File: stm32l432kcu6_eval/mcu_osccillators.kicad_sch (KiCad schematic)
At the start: 8 parts, among them U1 STM32L432KCUx, Y1 ASFL1-40.000MHZ-EC-T, Y2 FC-135_32.7680KA-A3

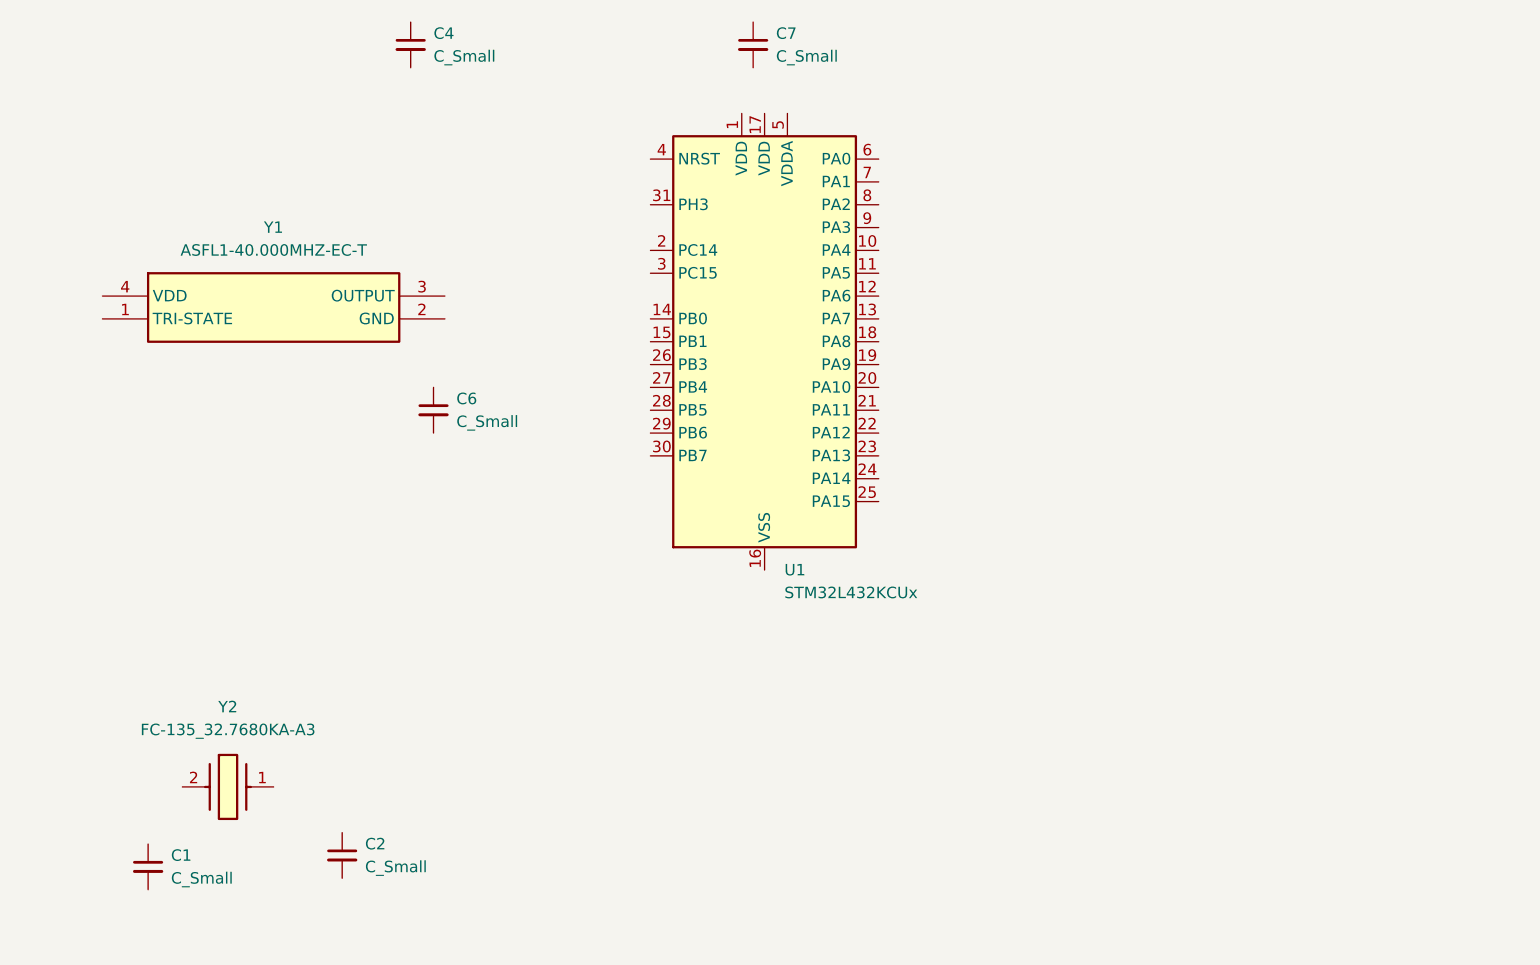
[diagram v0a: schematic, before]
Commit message: board save 1
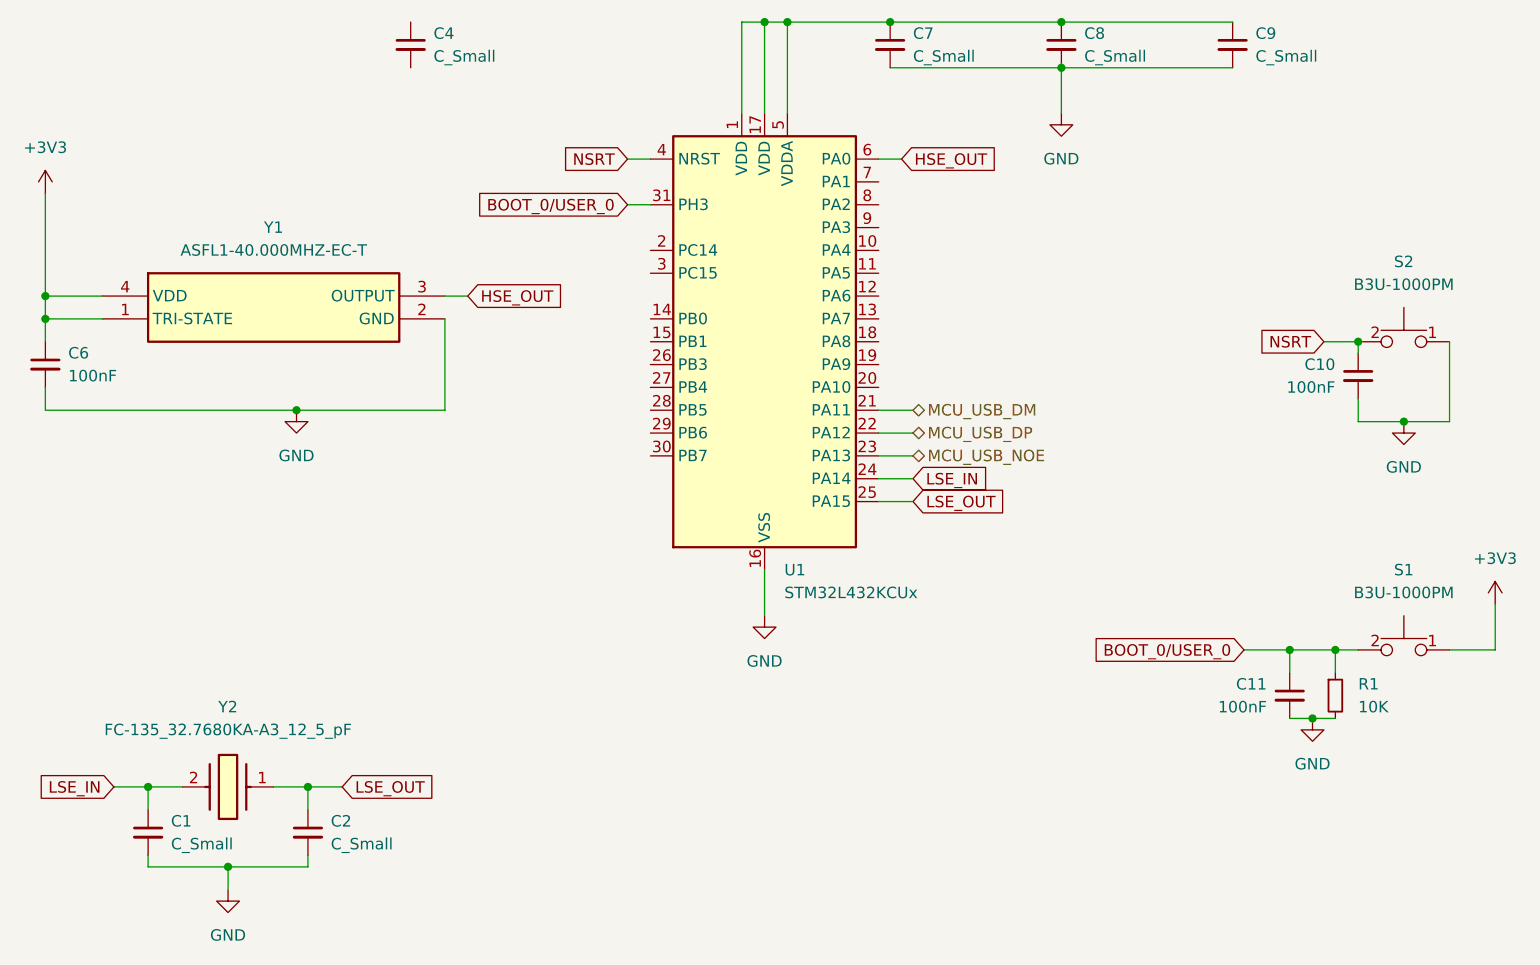
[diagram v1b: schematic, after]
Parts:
- added C10, C11: 100nF, Capacitor_SMD:C_0603_1608Metric, symbol Device:C_Small
- added C8, C9: C_Small, Capacitor_SMD:C_0603_1608Metric, symbol Device:C_Small
- added R1: 10K, Resistor_SMD:R_0603_1608Metric, symbol Device:R_Small
- added S1, S2: B3U-1000PM, custom_part_library_1:B3U1000PM_3D_MODEL, symbol B3U-1000PM_OMRON:B3U-1000PM
- C6: value C_Small -> 100nF
- Y2: value FC-135_32.7680KA-A3 -> FC-135_32.7680KA-A3_12_5_pF
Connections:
- net at U1.1 (VDD): now also C7.1, U1.17 (VDD), U1.5 (VDDA), C8.1, C9.1
- net GND: now reaches U1.16 (VSS), U1.32 (VSS), U1.33 (VSS)
- net GND: now also C1.2, C2.2, C6.2, C7.2, Y1.2 (GND), C10.2, C11.2, C8.2, C9.2, R1.2, S2.1
- net MCU_USB_DM: now reaches U1.21 (PA11)
- net MCU_USB_DP: now reaches U1.22 (PA12)
- net MCU_USB_NOE: now reaches U1.23 (PA13)
- net LSE_IN: now reaches U1.24 (PA14)
- net LSE_IN: now also C1.1, Y2.2 (X2)
- net LSE_OUT: now reaches U1.25 (PA15)
- net LSE_OUT: now also C2.1, Y2.1
- net BOOT_0/USER_0: now reaches U1.31 (PH3)
- net BOOT_0/USER_0: now also C11.1, R1.1, S1.2
- net NSRT: now reaches U1.4 (NRST)
- net NSRT: now also C10.1, S2.2
- net HSE_OUT: now reaches U1.6 (PA0)
- net HSE_OUT: now also Y1.3 (OUTPUT)
- net +3V3: now reaches C6.1
- net +3V3: now also Y1.1 (TRI-STATE), Y1.4 (VDD), S1.1
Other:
- moved on the sheet: C1, C2, C6, C7

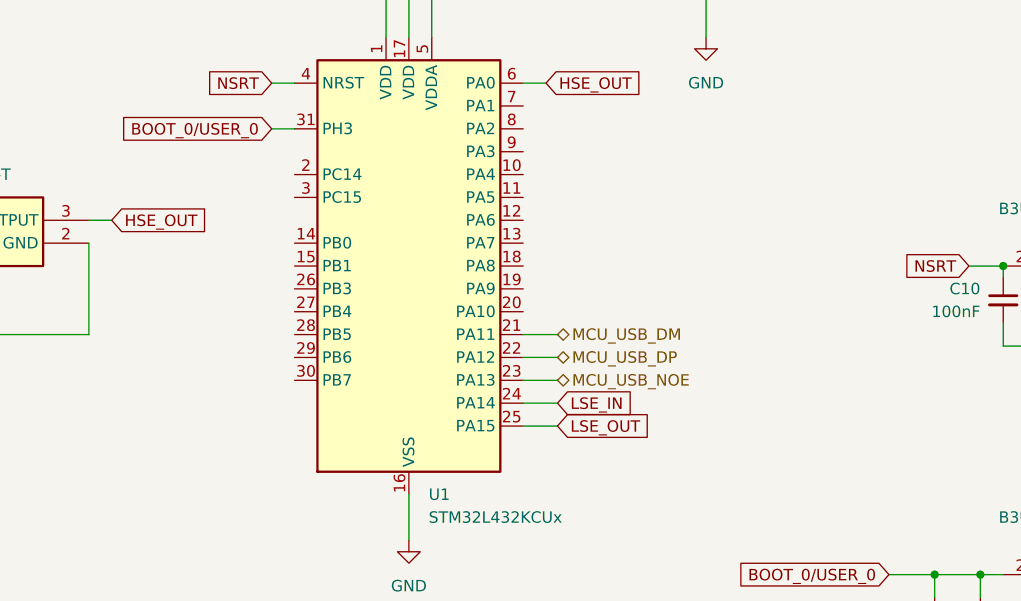
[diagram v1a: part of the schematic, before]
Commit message: board save 2
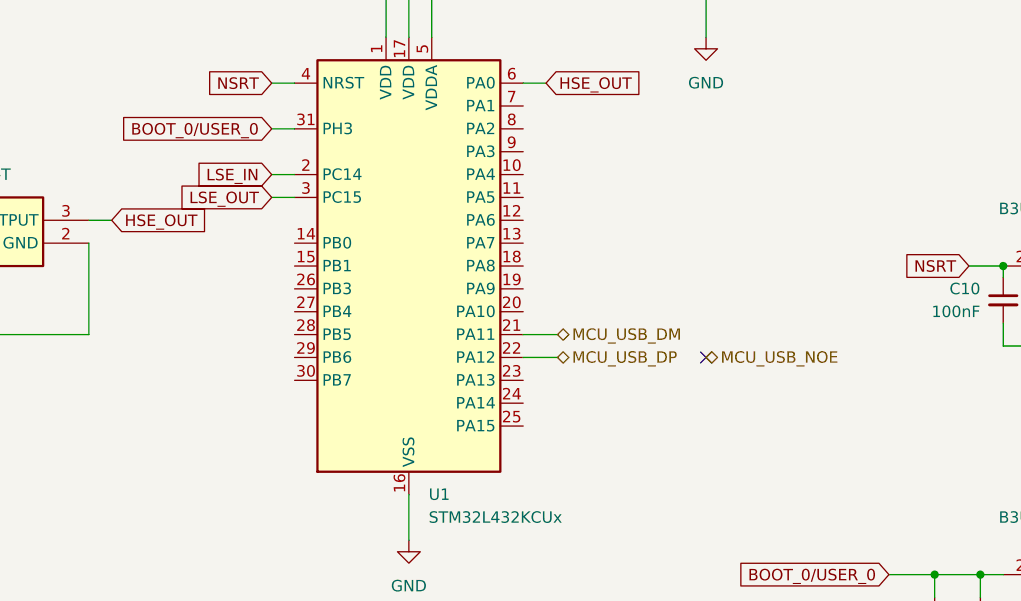
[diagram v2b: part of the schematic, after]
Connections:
- net LSE_IN: now also U1.2 (PC14); no longer U1.24 (PA14)
- net LSE_OUT: now also U1.3 (PC15); no longer U1.25 (PA15)
- net MCU_USB_NOE: no longer U1.23 (PA13)
- no-connect marks 0 -> 1
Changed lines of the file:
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@@
 		(color 0 0 0 0)
 	)
+	(no_connect
+		(at 220.98 90.17)
+	)
 	(wire
 		(pts
@@
 	(wire
 		(pts
-			(xy 200.66 92.71) (xy 204.47 92.71)
-		)
-		(stroke
-			(width 0)
-			(type default)
-		)
-	)
-	(wire
-		(pts
 			(xy 248.92 121.92) (xy 251.46 121.92)
 		)
@@
 	(wire
 		(pts
-			(xy 200.66 95.25) (xy 204.47 95.25)
-		)
-		(stroke
-			(width 0)
-			(type default)
-		)
-	)
-	(wire
-		(pts
 			(xy 241.3 114.3) (xy 246.38 114.3)
 		)
@@
 	(wire
 		(pts
+			(xy 172.72 69.85) (xy 175.26 69.85)
+		)
+		(stroke
+			(width 0)
+			(type default)
+		)
+	)
+	(wire
+		(pts
 			(xy 172.72 59.69) (xy 175.26 59.69)
 		)
@@
 	(wire
 		(pts
-			(xy 200.66 97.79) (xy 204.47 97.79)
+			(xy 172.72 72.39) (xy 175.26 72.39)
 		)
 		(stroke
@@
 	(global_label "LSE_IN"
 		(shape input)
-		(at 204.47 95.25 0)
+		(at 172.72 69.85 180)
+		(fields_autoplaced yes)
+		(effects
+			(font
+				(size 1.27 1.27)
+			)
+			(justify right)
+		)
+		(property "Intersheetrefs" "${INTERSHEET_REFS}"
+			(at 163.4453 69.85 0)
+			(effects
+				(font
+					(size 1.27 1.27)
+				)
+				(justify right)
+				(hide yes)
+			)
+		)
+	)
+	(global_label "NSRT"
+		(shape input)
+		(at 172.72 59.69 180)
+		(fields_autoplaced yes)
+		(effects
+			(font
+				(size 1.27 1.27)
+			)
+			(justify right)
+		)
+		(property "Intersheetrefs" "${INTERSHEET_REFS}"
+			(at 164.9572 59.69 0)
+			(effects
+				(font
+					(size 1.27 1.27)
+				)
+				(justify right)
+				(hide yes)
+			)
+		)
+	)
+	(global_label "NSRT"
+		(shape input)
+		(at 250.19 80.01 180)
+		(fields_autoplaced yes)
+		(effects
+			(font
+				(size 1.27 1.27)
+			)
+			(justify right)
+		)
+		(property "Intersheetrefs" "${INTERSHEET_REFS}"
+			(at 242.4272 80.01 0)
+			(effects
+				(font
+					(size 1.27 1.27)
+				)
+				(justify right)
+				(hide yes)
+			)
+		)
+	)
+	(global_label "BOOT_0{slash}USER_0"
+		(shape input)
+		(at 241.3 114.3 180)
+		(fields_autoplaced yes)
+		(effects
+			(font
+				(size 1.27 1.27)
+			)
+			(justify right)
+		)
+		(property "Intersheetrefs" "${INTERSHEET_REFS}"
+			(at 222.7725 114.3 0)
+			(effects
+				(font
+					(size 1.27 1.27)
+				)
+				(justify right)
+				(hide yes)
+			)
+		)
+	)
+	(global_label "HSE_OUT"
+		(shape input)
+		(at 154.94 74.93 0)
 		(fields_autoplaced yes)
 		(effects
@@
 		)
 		(property "Intersheetrefs" "${INTERSHEET_REFS}"
-			(at 213.7447 95.25 0)
+			(at 166.2104 74.93 0)
 			(effects
 				(font
@@
 		)
 	)
-	(global_label "NSRT"
-		(shape input)
-		(at 172.72 59.69 180)
+	(global_label "LSE_OUT"
+		(shape input)
+		(at 172.72 72.39 180)
 		(fields_autoplaced yes)
 		(effects
@@
 		)
 		(property "Intersheetrefs" "${INTERSHEET_REFS}"
-			(at 164.9572 59.69 0)
+			(at 161.752 72.39 0)
 			(effects
 				(font
@@
 				)
 				(justify right)
-				(hide yes)
-			)
-		)
-	)
-	(global_label "NSRT"
-		(shape input)
-		(at 250.19 80.01 180)
-		(fields_autoplaced yes)
-		(effects
-			(font
-				(size 1.27 1.27)
-			)
-			(justify right)
-		)
-		(property "Intersheetrefs" "${INTERSHEET_REFS}"
-			(at 242.4272 80.01 0)
-			(effects
-				(font
-					(size 1.27 1.27)
-				)
-				(justify right)
-				(hide yes)
-			)
-		)
-	)
-	(global_label "BOOT_0{slash}USER_0"
-		(shape input)
-		(at 241.3 114.3 180)
-		(fields_autoplaced yes)
-		(effects
-			(font
-				(size 1.27 1.27)
-			)
-			(justify right)
-		)
-		(property "Intersheetrefs" "${INTERSHEET_REFS}"
-			(at 222.7725 114.3 0)
-			(effects
-				(font
-					(size 1.27 1.27)
-				)
-				(justify right)
-				(hide yes)
-			)
-		)
-	)
-	(global_label "HSE_OUT"
-		(shape input)
-		(at 154.94 74.93 0)
-		(fields_autoplaced yes)
-		(effects
-			(font
-				(size 1.27 1.27)
-			)
-			(justify left)
-		)
-		(property "Intersheetrefs" "${INTERSHEET_REFS}"
-			(at 166.2104 74.93 0)
-			(effects
-				(font
-					(size 1.27 1.27)
-				)
-				(justify left)
-				(hide yes)
-			)
-		)
-	)
-	(global_label "LSE_OUT"
-		(shape input)
-		(at 204.47 97.79 0)
-		(fields_autoplaced yes)
-		(effects
-			(font
-				(size 1.27 1.27)
-			)
-			(justify left)
-		)
-		(property "Intersheetrefs" "${INTERSHEET_REFS}"
-			(at 215.438 97.79 0)
-			(effects
-				(font
-					(size 1.27 1.27)
-				)
-				(justify left)
 				(hide yes)
 			)
@@
 	(hierarchical_label "MCU_USB_NOE"
 		(shape bidirectional)
-		(at 204.47 92.71 0)
-		(fields_autoplaced yes)
-		(effects
+		(at 220.98 90.17 0)
+		(fields_autoplaced yes)
+		(effects

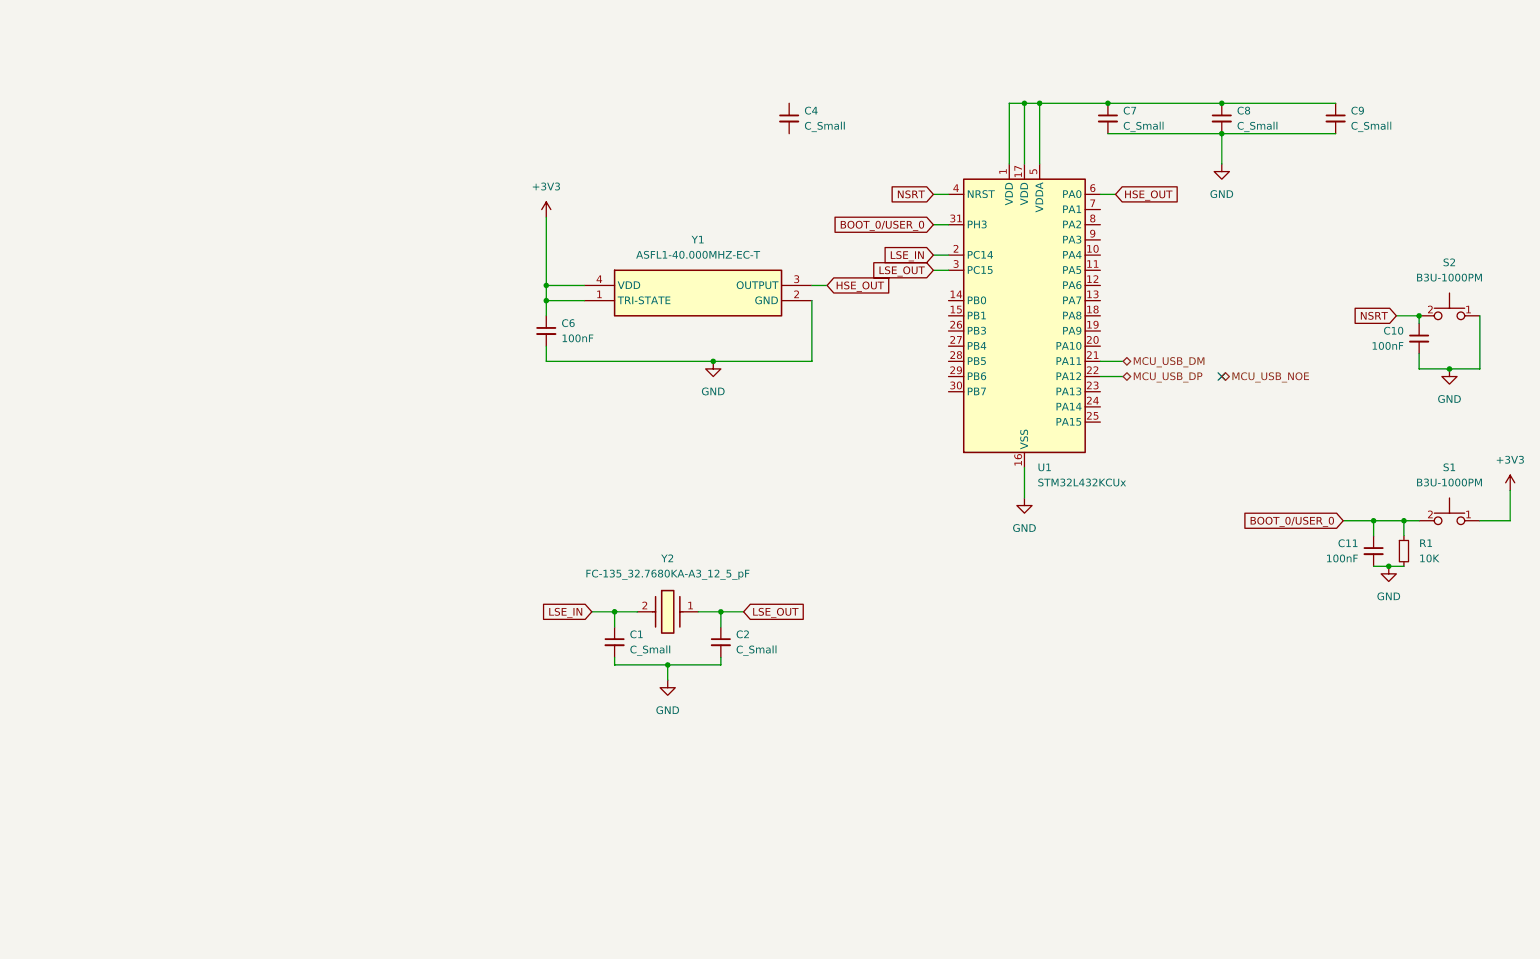
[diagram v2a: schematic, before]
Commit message: board save 4
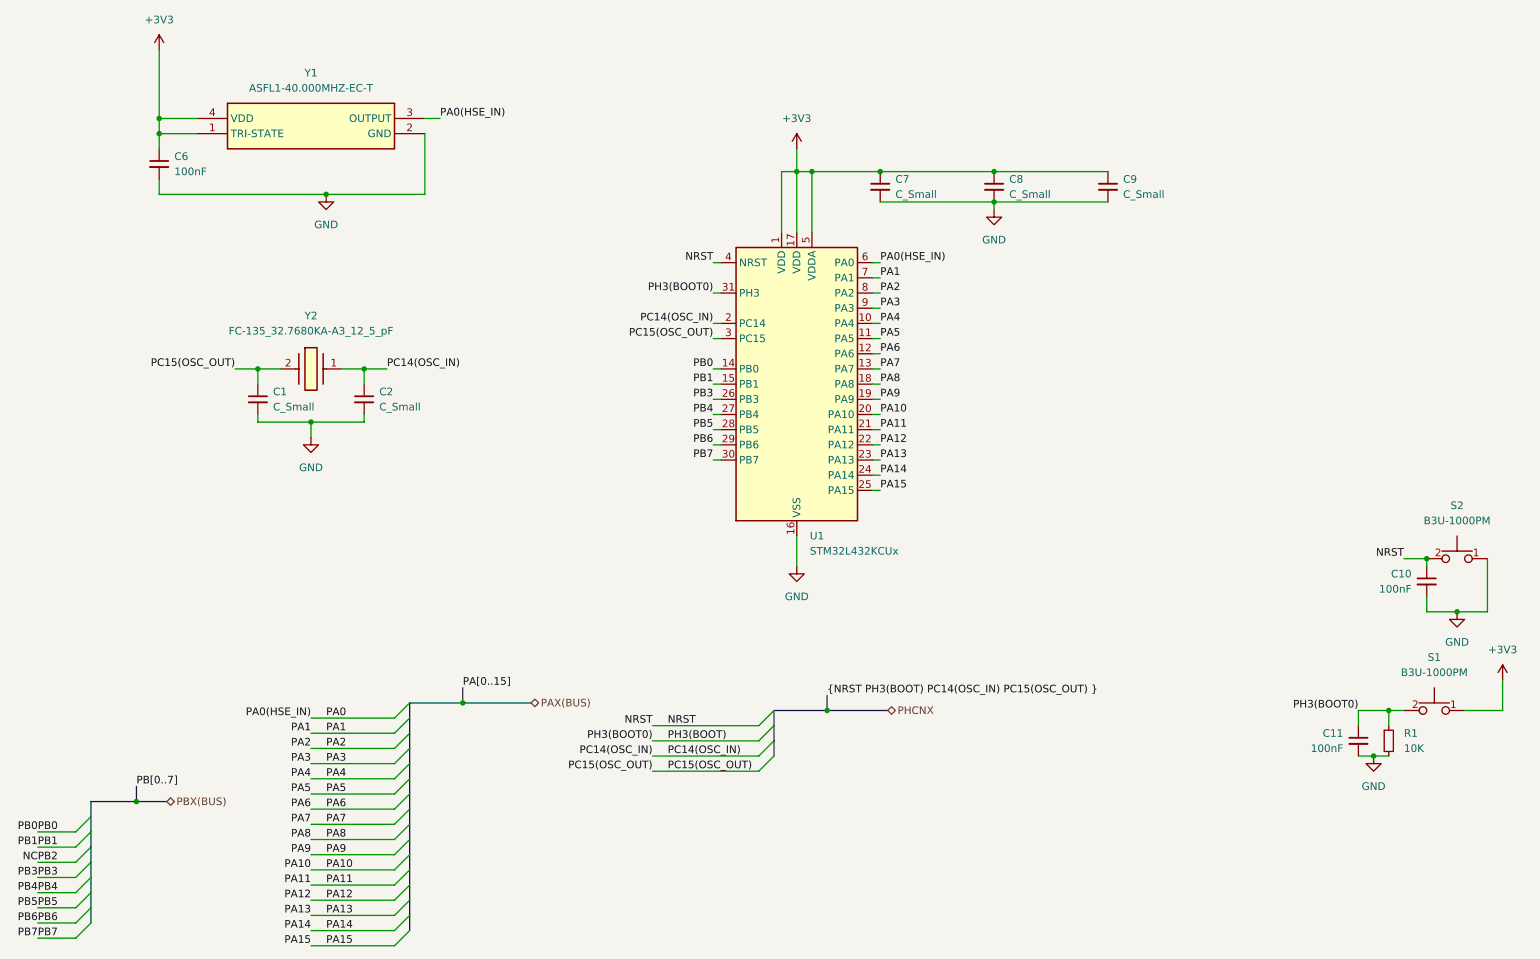
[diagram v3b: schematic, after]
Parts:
- removed C4: C_Small, Capacitor_SMD:C_0603_1608Metric, symbol Device:C_Small
- Y2: footprint FC135327680KAA3 -> FC_135_CLOCK_KI_CAD:FC-135_32_7680KA-A3
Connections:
- net +3V3: now also C7.1, C8.1, C9.1, U1.1 (VDD), U1.17 (VDD), U1.5 (VDDA)
- net PA4: now reaches U1.10 (PA4)
- net PA5: now reaches U1.11 (PA5)
- net PA6: now reaches U1.12 (PA6)
- net PA7: now reaches U1.13 (PA7)
- net PB0: now reaches U1.14 (PB0)
- net PB1: now reaches U1.15 (PB1)
- net PA8: now reaches U1.18 (PA8)
- net PA9: now reaches U1.19 (PA9)
- net PA10: now reaches U1.20 (PA10)
- net PA13: now reaches U1.23 (PA13)
- net PA14: now reaches U1.24 (PA14)
- net PA15: now reaches U1.25 (PA15)
- net PB3: now reaches U1.26 (PB3)
- net PB4: now reaches U1.27 (PB4)
- net PB5: now reaches U1.28 (PB5)
- net PB6: now reaches U1.29 (PB6)
- net PB7: now reaches U1.30 (PB7)
- net PA1: now reaches U1.7 (PA1)
- net PA2: now reaches U1.8 (PA2)
- net PA3: now reaches U1.9 (PA3)
- net BOOT_0/USER_0 renamed PH3(BOOT)
- net HSE_OUT renamed PA0
- net LSE_IN renamed PC15(OSC_OUT)
- net PC15(OSC_OUT): now also U1.3 (PC15); no longer U1.2 (PC14)
- net LSE_OUT renamed PC14(OSC_IN)
- net PC14(OSC_IN): now also U1.2 (PC14); no longer U1.3 (PC15)
- net MCU_USB_DM renamed PA11
- net MCU_USB_DP renamed PA12
- net NSRT renamed NRST
- no-connect marks 1 -> 0
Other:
- moved on the sheet: C1, C10, C11, C2, C6, C7, C8, C9, R1, S1, S2, U1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
